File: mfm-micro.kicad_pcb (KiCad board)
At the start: 2 copper layers, 57 x 34 mm, 66 parts, among them J1 USB, P1 Peripheral1_connector, P2 Peripheral2_connector, Q1 AO3401A, U1 USBLC6-2P6, U2 TP4056, U3 XC6206P332MR, U4 STM32L072CBTx

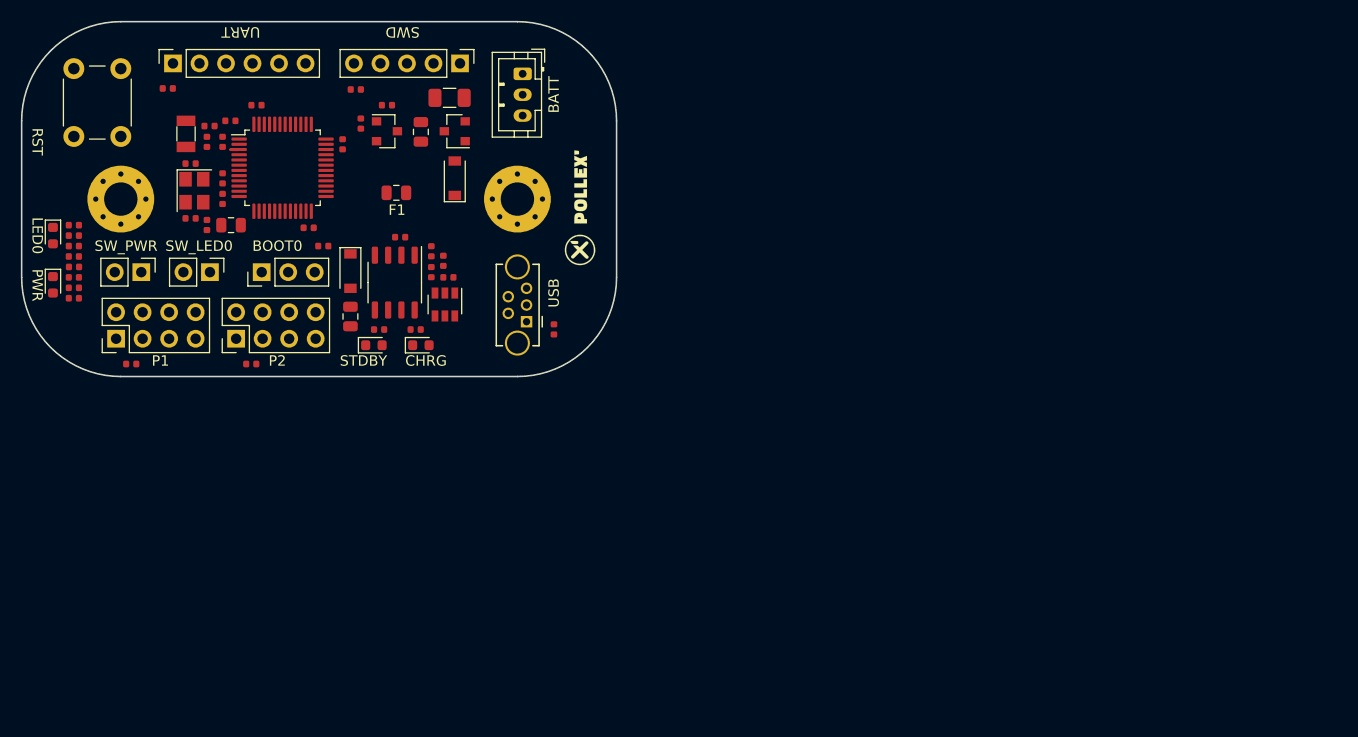
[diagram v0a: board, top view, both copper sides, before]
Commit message: Rerout and new exports
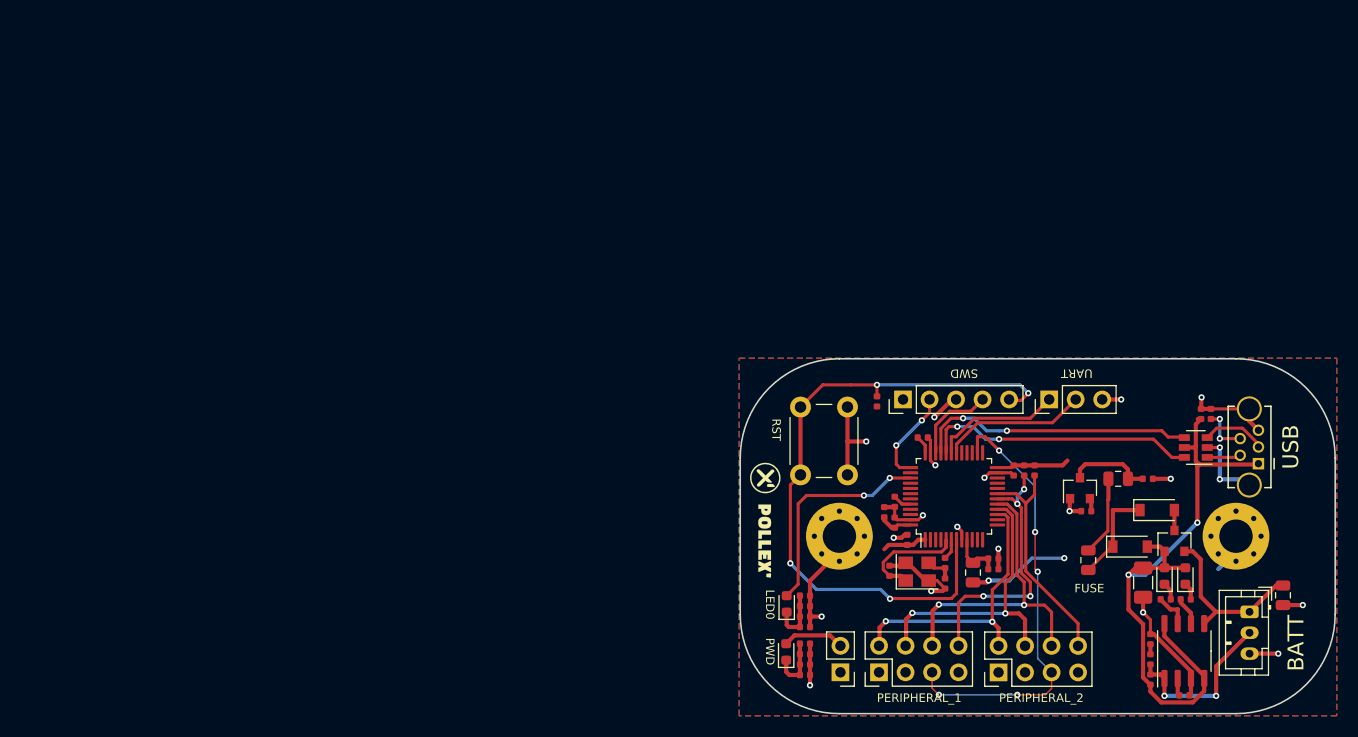
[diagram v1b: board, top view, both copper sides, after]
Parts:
- removed BATT: JST PH 3, Connector_JST:JST_PH_B3B-PH-K_1x03_P2.00mm_Vertical
- removed BOOT0: SW_DPDT_x2, Connector_PinHeader_2.54mm:PinHeader_1x03_P2.54mm_Vertical
- removed C14, C15: 12p, Capacitor_SMD:C_0402_1005Metric
- removed C17: 100n, Capacitor_SMD:C_0402_1005Metric
- removed CHRG, PWR: Red, LED_SMD:LED_0603_1608Metric
- removed LED0, STDBY: Green, LED_SMD:LED_0603_1608Metric
- removed R22: 130, Resistor_SMD:R_0402_1005Metric
- removed RST: SW_RST, Button_Switch_THT:SW_PUSH_6mm
- removed SWD: SWD_connector, Connector_PinHeader_2.54mm:PinHeader_1x05_P2.54mm_Vertical
- removed SW_LED0: STAT_LED_Switch, Connector_PinHeader_2.54mm:PinHeader_1x02_P2.54mm_Vertical
- removed SW_PWR: PWR_LED_Switch, Connector_PinHeader_2.54mm:PinHeader_1x02_P2.54mm_Vertical
- removed UART: UART_Connector, Connector_PinSocket_2.54mm:PinSocket_1x06_P2.54mm_Vertical
- removed XOSC32: 32.768KHz, Crystal:Crystal_SMD_3215-2Pin_3.2x1.5mm
- added D2: Green, LED_SMD:LED_0603_1608Metric, F.Cu at (157.0, 102.6)
- added D3: Red, LED_SMD:LED_0603_1608Metric, F.Cu at (155.0, 102.6)
- added D5: Green, LED_SMD:LED_0603_1608Metric, F.Cu at (118.8, 105.3)
- added D6: Red, LED_SMD:LED_0603_1608Metric, F.Cu at (118.8, 109.9)
- added J2: JST PH 3, Connector_JST:JST_PH_B3B-PH-K_1x03_P2.00mm_Vertical, F.Cu at (163.2, 106.0)
- added J3: SWD_connector, Connector_PinHeader_2.54mm:PinHeader_1x05_P2.54mm_Vertical, F.Cu at (129.9, 85.7)
- added J4: Conn_01x03, Connector_PinHeader_2.54mm:PinHeader_1x03_P2.54mm_Vertical, F.Cu at (143.9, 85.7)
- added R14: 130, Resistor_SMD:R_0402_1005Metric, F.Cu at (120.5, 105.5)
- added REF**: OSHW-Logo2_7.3x6mm_SilkScreen, Symbol:OSHW-Logo2_7.3x6mm_SilkScreen, B.Cu at (152.8, 110.2)
- added SW1: SW_RST, Button_Switch_THT:SW_PUSH_6mm, F.Cu at (124.6, 86.4)
- added SW4: PWR_LED_Switch, Connector_PinHeader_2.54mm:PinHeader_1x02_P2.54mm_Vertical, F.Cu at (124.0, 111.8)
- C1: value 1u -> 4.7u
- C12, C13: value 20p -> 12p
- C3: value 4.7u -> 1u
- J1: value USB -> USB_B_Mini
- R10: value 10k -> 680
- R12: value 10k -> 130
- R16: value 680 -> 130
- R20, R21: value 130 -> 10k
- U1: value USBLC6-2P6 -> XC6206P332MR; footprint Package_TO_SOT_SMD:SOT-23-6 -> Package_TO_SOT_SMD:SOT-23
- U3: value XC6206P332MR -> USBLC6-2P6; footprint Package_TO_SOT_SMD:SOT-23 -> Package_TO_SOT_SMD:SOT-23-6
- moved R21 93.9 mm to (142.6, 92.5), turned to 270 degrees
- moved C4 93.3 mm to (166.3, 104.5), turned to 270 degrees
- moved R20 92.7 mm to (141.6, 92.5), turned to 270 degrees
- moved R8 87.0 mm to (156.9, 114.0), turned to 180 degrees
- moved U2 83.5 mm to (156.9, 109.8), turned to 90 degrees
- moved C1 83.4 mm to (158.5, 87.1), turned to 90 degrees
- moved U3 83.2 mm to (158.0, 90.3), turned to 180 degrees
- moved C10 82.8 mm to (138.6, 102.0), turned to 0 degrees
- moved C2 82.7 mm to (153.4, 93.3), turned to 0 degrees
- moved C13 82.4 mm to (134.0, 103.3), turned to 270 degrees
- moved C7 82.1 mm to (140.6, 92.5)
- moved C11 81.8 mm to (138.6, 101.0), turned to 0 degrees
- moved R5 81.5 mm to (157.0, 104.8), turned to 180 degrees
- moved R1 81.1 mm to (152.9, 103.2), turned to 270 degrees
- moved R19 80.7 mm to (120.5, 109.1)
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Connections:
- net SPI_SS3 renamed Net-(U4-Pad20)
- C1 pad 1: Net-(C1-Pad1) -> VBUS
- C12 pad 1: XOSC32_IN -> XOSC_IN
- C13 pad 1: XOSC32_OUT -> Net-(C13-Pad1)
- C2 pad 1: +3V3 -> Net-(C2-Pad1)
- C3 pad 1: VBUS -> +3V3
- FB1 pad 2: Net-(C1-Pad1) -> Net-(C2-Pad1)
- J1 pad 2: D- -> USB_CONN_D-
- J1 pad 3: D+ -> USB_CONN_D+
- P1 pad 3: SPI_SS1 -> GND
- P1 pad 5: GND -> P_EXTI
- P1 pad 7: P_EXTI -> Net-(P1-Pad7)
- P1 pad 8: Net-(J3-Pad8) -> SPI_SS1
- P2 pad 3: SPI_SS2 -> GND
- P2 pad 5: GND -> P_EXTI
- P2 pad 7: P_EXTI -> Net-(P2-Pad7)
- P2 pad 8: Net-(J5-Pad8) -> SPI_SS2
- R10 pad 1: BOOT0 -> Net-(C13-Pad1)
- R10 pad 2: Net-(R10-Pad2) -> XOSC_OUT
- R11 pad 1: +3V3 -> BOOT0
- R11 pad 2: SPI_SS1 -> GND
- R12 pad 1: +3V3 -> GND
- R12 pad 2: SPI_SS2 -> Net-(D5-Pad1)
- R15 pad 2: Net-(D6-Pad1) -> Net-(D5-Pad1)
- R16 pad 1: Net-(C15-Pad1) -> GND
- R16 pad 2: XOSC_OUT -> Net-(D6-Pad1)
- R17 pad 2: Net-(D5-Pad1) -> Net-(D6-Pad1)
- R18 pad 2: Net-(D5-Pad1) -> Net-(D6-Pad1)
- R19 pad 2: Net-(D5-Pad1) -> Net-(D6-Pad1)
- R20 pad 1: GND -> +3V3
- R20 pad 2: Net-(D6-Pad1) -> SPI_SS1
- R21 pad 1: GND -> +3V3
- R21 pad 2: Net-(D6-Pad1) -> SPI_SS2
- U1 pad 1: USB_DM -> GND
- U1 pad 2: GND -> +3V3
- U1 pad 3: USB_DP -> Net-(C2-Pad1)
- U3 pad 1: GND -> USB_CONN_D-
- U3 pad 2: +3V3 -> GND
- U3 pad 3: Net-(C1-Pad1) -> USB_CONN_D+
- U4 pad 26: LED0 -> P_EXTI
- U4 pad 3: XOSC32_IN -> Net-(U4-Pad3)
- U4 pad 32: USB_DM -> USB_D-
- U4 pad 33: USB_DP -> USB_D+
- U4 pad 39: P_EXTI -> LED0
- U4 pad 4: XOSC32_OUT -> Net-(U4-Pad4)
- XOSC1 pad 3: Net-(C15-Pad1) -> Net-(C13-Pad1)
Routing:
- net GND: track 0.00 -> 98.3 mm, vias 0 -> 20
- net NRST: track 0.00 -> 64.4 mm, vias 0 -> 4
- net VBUS: track 0.00 -> 61.5 mm, vias 0 -> 2
- net P_EXTI: track 0.00 -> 42.6 mm, vias 0 -> 5
- net SPI_MOSI: track 0.00 -> 29.8 mm, vias 0 -> 2
- net SPI_MISO: track 0.00 -> 28.5 mm, vias 0 -> 2
- net +3V3: track 0.00 -> 28.1 mm, vias 0 -> 2
- net SPI_SCK: track 0.00 -> 27.1 mm, vias 0 -> 2
- net USB_D+: track 0.00 -> 26.8 mm, vias 0 -> 2
- net USB_D-: track 0.00 -> 26.5 mm, vias 0 -> 2
- net SPI_SS1: track 0.00 -> 25.8 mm, vias 0 -> 4
- net SPI_SS2: track 0.00 -> 21.9 mm
- net LED0: track 0.00 -> 21.0 mm, vias 0 -> 2
- net +BATT: track 0.00 -> 16.6 mm
- net BATT_T: track 0.00 -> 16.5 mm, vias 0 -> 2
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- added copper zone on F.Cu, net +3V3
- added copper zone on B.Cu, net GND
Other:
- copper layers 2 -> 4
- net class Default: clearance 0.2 -> 0.127; trace_width 0.25 -> 0.127; via_dia 0.8 -> 0.6; via_drill 0.4 -> 0.3
- rule pad_to_mask_clearance: 0.05 -> 0
- rule trace_clearance: 0.2 -> 0.127
- rule trace_min: 0.2 -> 0.127
- rule via_min_size: 0.4 -> 0.6
- board text added: "BATT"
- board text added: "FUSE"
- board text added: "LED0"
- board text added: "MFM Micro V0.1 Prototype Board"
- board text added: "PERIPHERAL_1"
- board text added: "PERIPHERAL_2"
- board text added: "PWD"
- board text added: "RST"
- board text added: "SWD"
- board text added: "UART"
- board text added: "USB"
- board text removed: "DTR"
- board text removed: "MFM Micro Prototype v0.1"
- board text removed: "NC"
- board text removed: "NRST"
